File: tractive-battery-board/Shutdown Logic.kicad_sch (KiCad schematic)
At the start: 31 parts, among them J10 Shutdown IL, K1 G6SK-2G, K2 G6DN-1A, K3 G6SK-2G, K4 G6DN-1A, U12 SN74HCS14DR, U13 SN74HCS08DR, U14 SZNUD3124DMT1G, U15 SZNUD3124DMT1G, U9 MCP6004

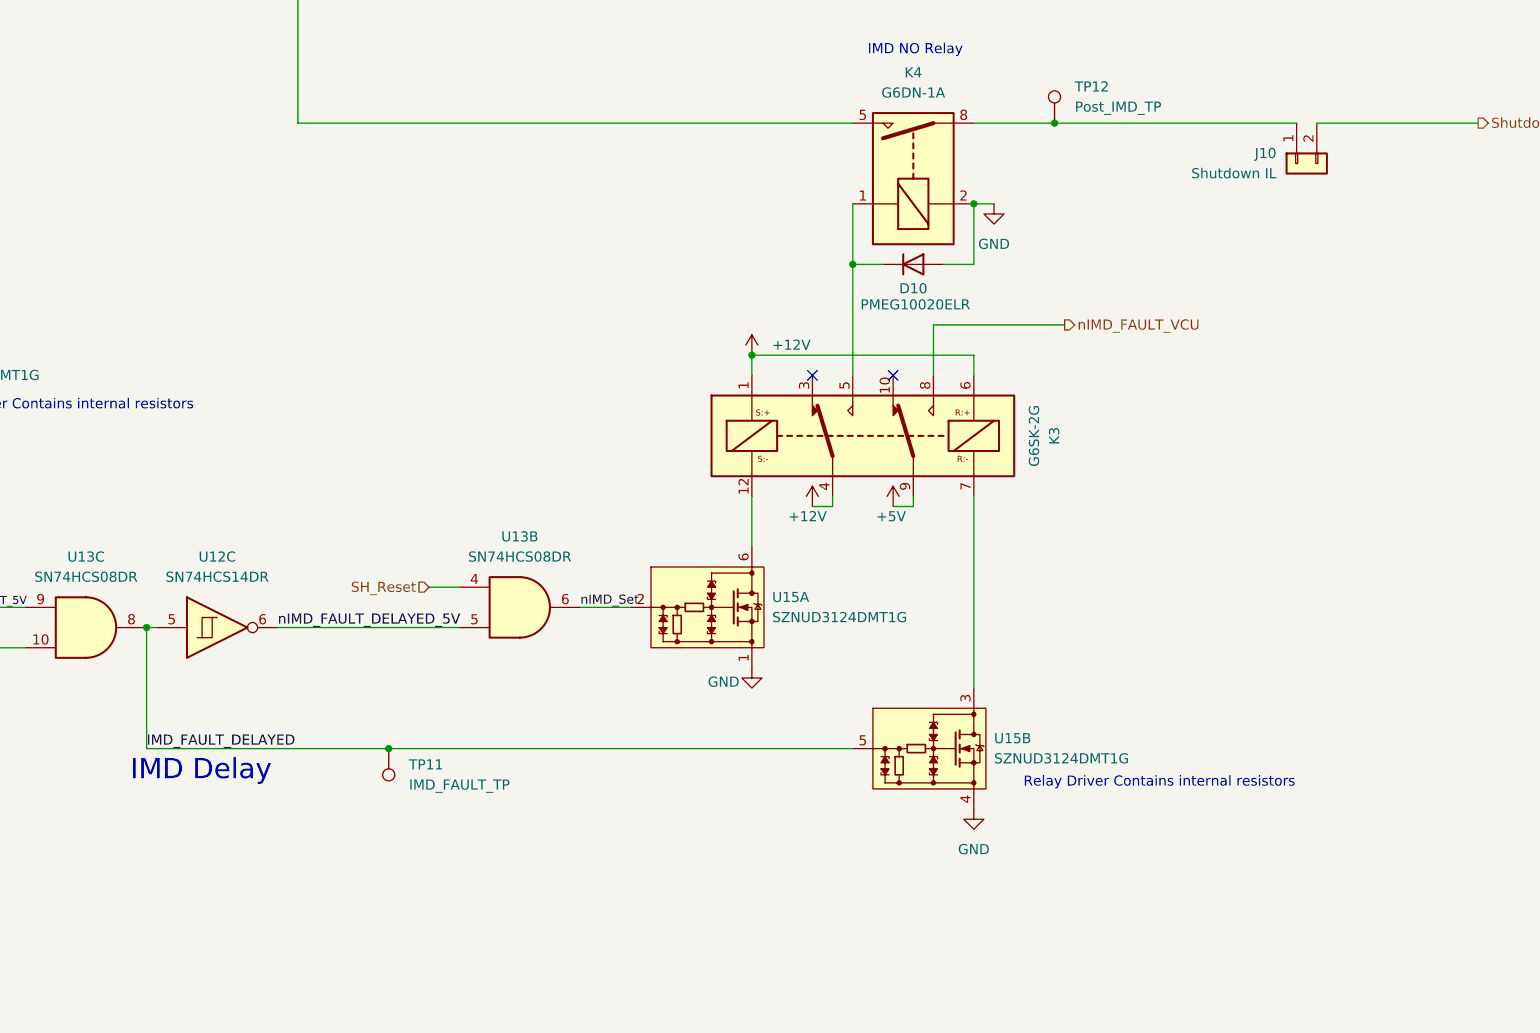
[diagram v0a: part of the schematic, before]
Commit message: IMD reset fix
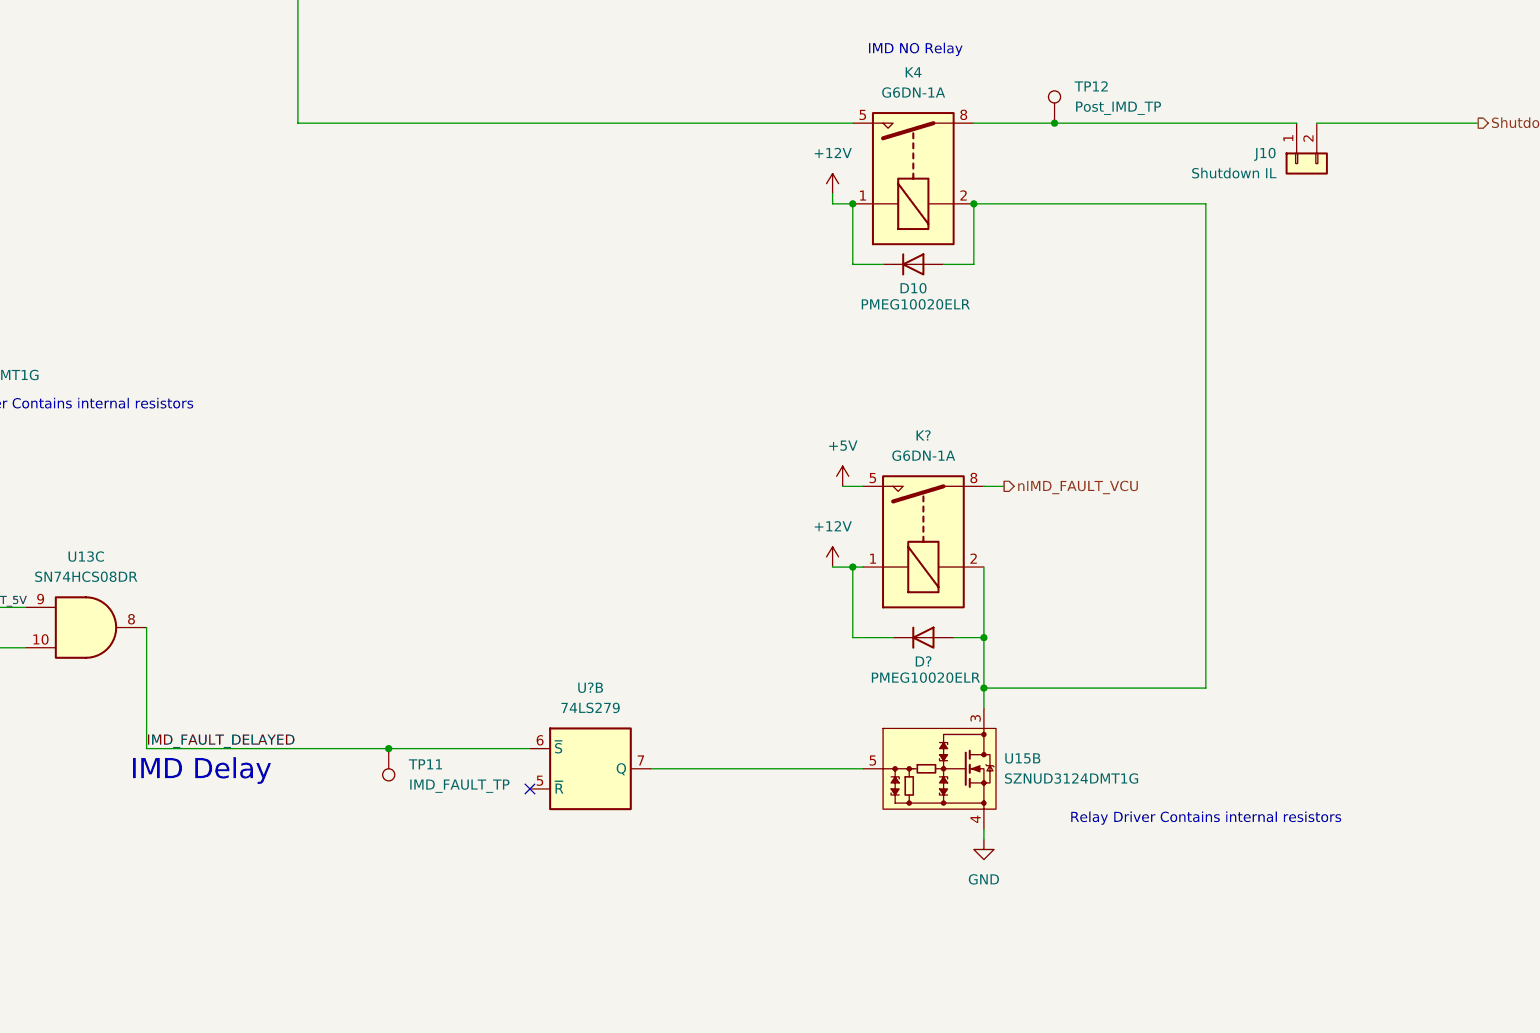
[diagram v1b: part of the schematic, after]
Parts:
- removed K3: G6SK-2G, Relay_SMD:Relay_DPDT_Omron_G6SK-2G, symbol Relay:G6SK-2
- removed unit 3 of U12
- removed unit 2 of U13
- removed unit 1 of U15
- added D?: PMEG10020ELR, Diode_SMD:Nexperia_CFP3_SOD-123W, symbol Device:D
- added K?: G6DN-1A, FS_4_Global_Footprint_Library:RELAY_G6DN-1A, symbol FS_4_Global_Symbol_Library:G6DN-1A
- added U?: 74LS279, symbol 74xx:74LS279
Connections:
- net +12V: now also D10.1 (K), K4.1, D?.1 (K), K?.1
- net +5V: now also K?.5
- net GND: no longer D10.2 (A), K4.2
- net IMD_FAULT_DELAYED: now also U?.6 (~{S}); no longer U15.5
- net nIMD_FAULT_VCU: now also K?.8
- net at U15.3: now also D10.2 (A), K4.2, D?.2 (A), K?.2
- new net: U15.5, U?.7 (Q)
- no-connect marks 4 -> 3
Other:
- moved on the sheet: U15B
